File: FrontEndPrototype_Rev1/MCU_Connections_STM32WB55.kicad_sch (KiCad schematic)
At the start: 2 parts, among them J1 Conn_02x19_Odd_Even, J2 Conn_02x19_Odd_Even

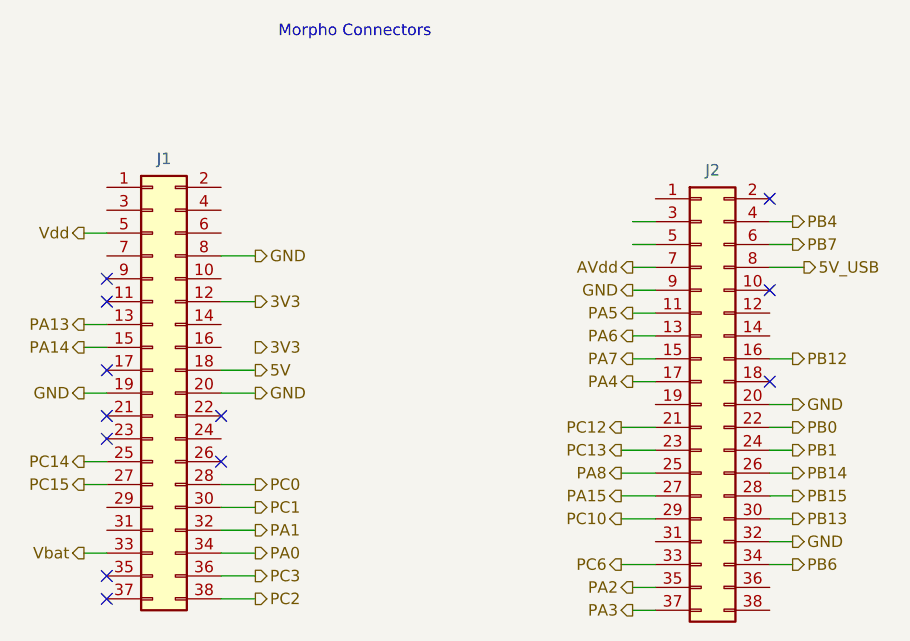
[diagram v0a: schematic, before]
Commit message: First Pass Schematic Fixes for Power Management Board
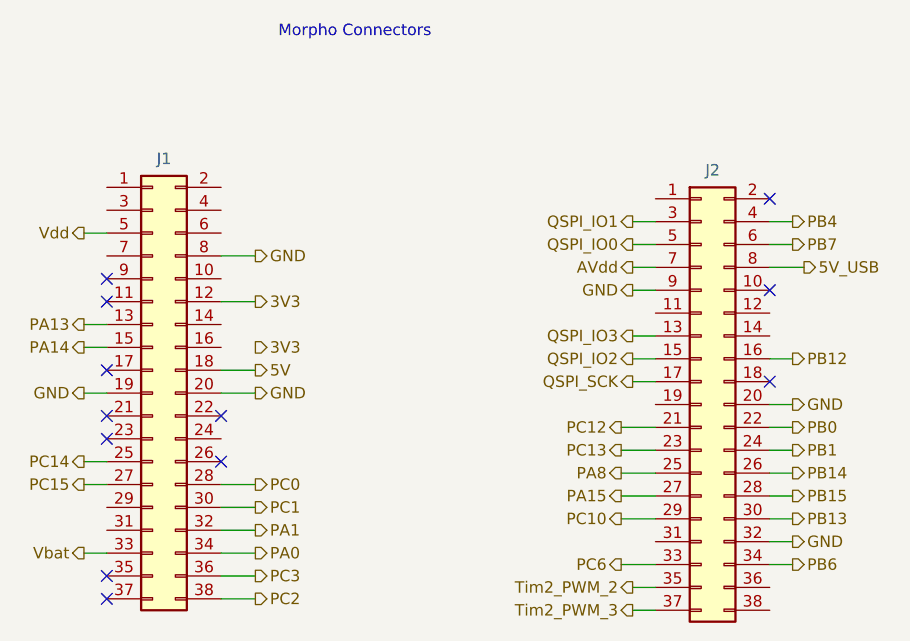
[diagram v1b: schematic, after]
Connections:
- net QSPI_IO1: now reaches J2.3 (Pin_3)
- net QSPI_IO0: now reaches J2.5 (Pin_5)
- net PA2 renamed Tim2_PWM_2
- net PA3 renamed Tim2_PWM_3
- net PA4 renamed QSPI_SCK
- net PA5: no longer names the net of J2.11 (Pin_11)
- net PA6 renamed QSPI_IO3
- net PA7 renamed QSPI_IO2

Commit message: Updated Measurement Board with new 3V Reference
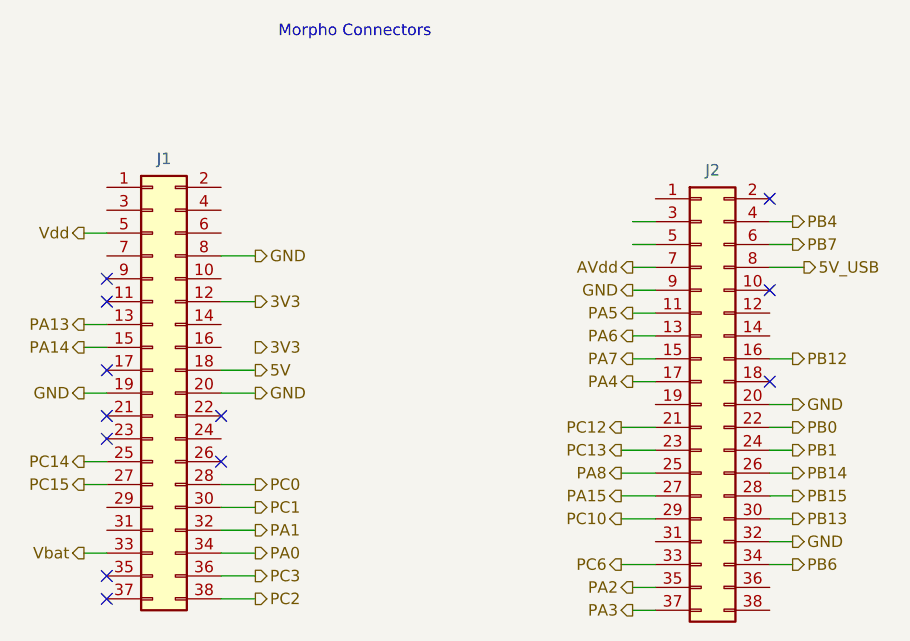
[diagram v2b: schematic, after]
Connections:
- net PA5: now reaches J2.11 (Pin_11)
- net QSPI_IO0: no longer names the net of J2.5 (Pin_5)
- net QSPI_IO1: no longer names the net of J2.3 (Pin_3)
- net QSPI_IO2 renamed PA7
- net QSPI_IO3 renamed PA6
- net QSPI_SCK renamed PA4
- net Tim2_PWM_2 renamed PA2
- net Tim2_PWM_3 renamed PA3
